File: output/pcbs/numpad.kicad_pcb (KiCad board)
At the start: 2 copper layers, 76 x 76 mm, 31 parts

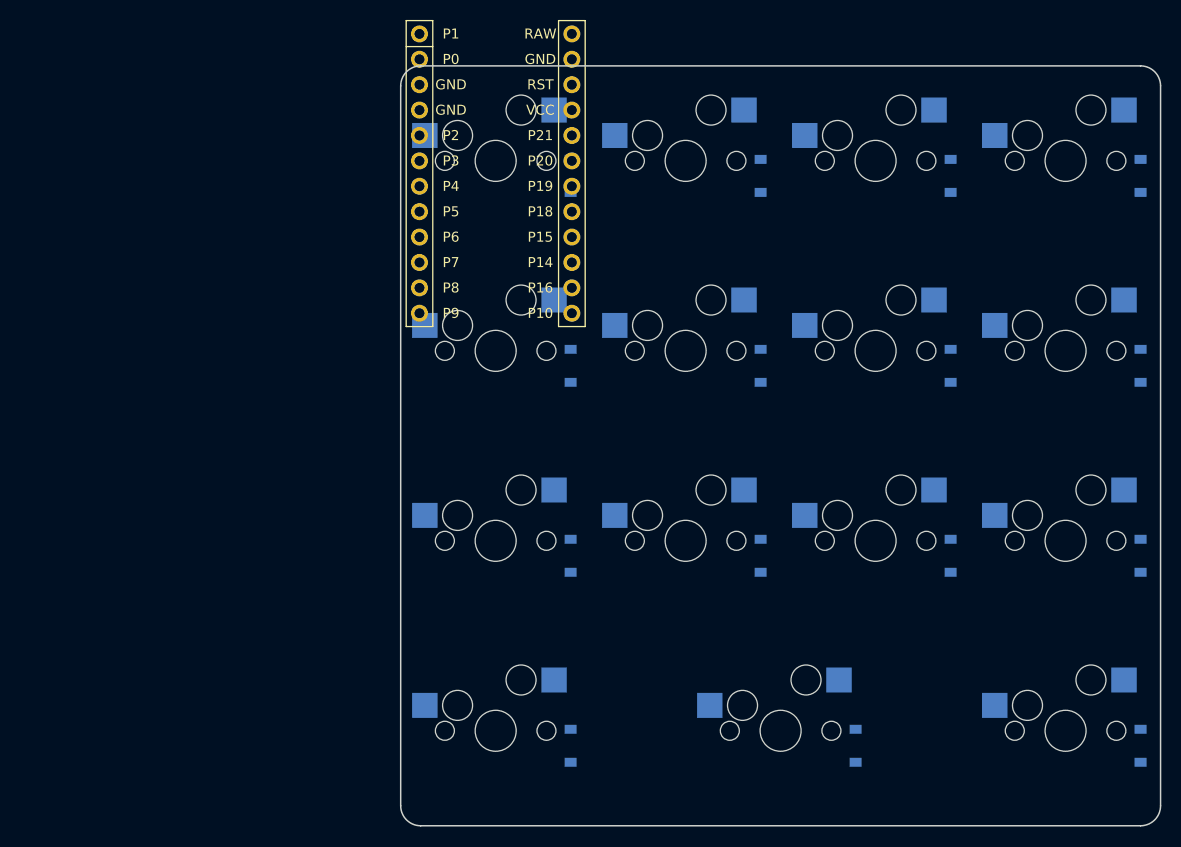
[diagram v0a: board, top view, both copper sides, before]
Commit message: build deley
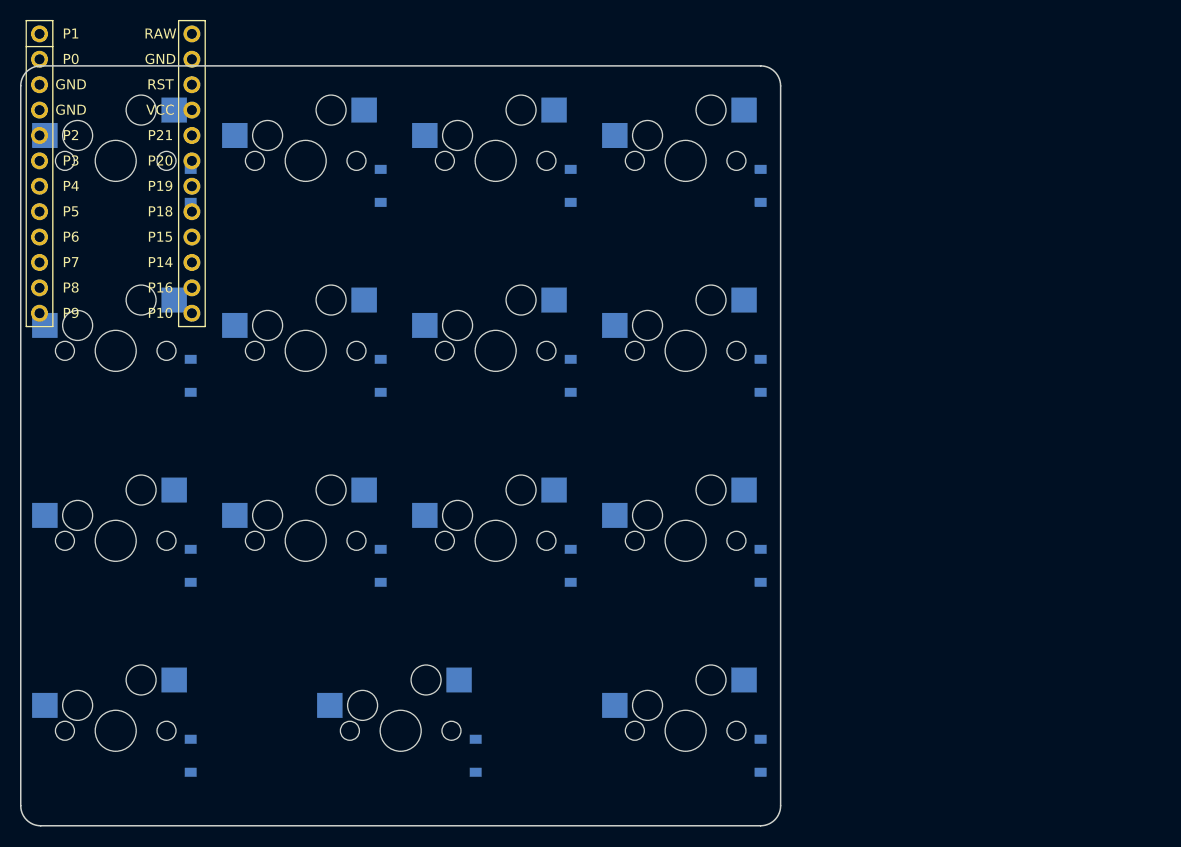
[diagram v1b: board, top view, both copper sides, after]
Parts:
- moved D1 38.0 mm to (22.5, 172.5)
- moved D10 38.0 mm to (60.5, 134.5)
- moved D11 38.0 mm to (60.5, 115.5)
- moved D12 38.0 mm to (79.5, 172.5)
- moved D13 38.0 mm to (79.5, 153.5)
- moved D14 38.0 mm to (79.5, 134.5)
- moved D15 38.0 mm to (79.5, 115.5)
- moved D2 38.0 mm to (22.5, 153.5)
- moved D3 38.0 mm to (22.5, 134.5)
- moved D4 38.0 mm to (22.5, 115.5)
- moved D5 38.0 mm to (51.0, 172.5)
- moved D6 38.0 mm to (41.5, 153.5)
- moved D7 38.0 mm to (41.5, 134.5)
- moved D8 38.0 mm to (41.5, 115.5)
- moved D9 38.0 mm to (60.5, 153.5)
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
